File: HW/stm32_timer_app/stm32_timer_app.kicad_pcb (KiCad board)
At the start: 2 copper layers, 121.5 x 72 mm, 30 parts, among them J1 105164-0001, J2 61300411121, J3 PH2-06-UA, Q1 BTA10-600BRG, U1 RT9193-33GB, U2 MOC3041SM, U3 STM32F103C8T6

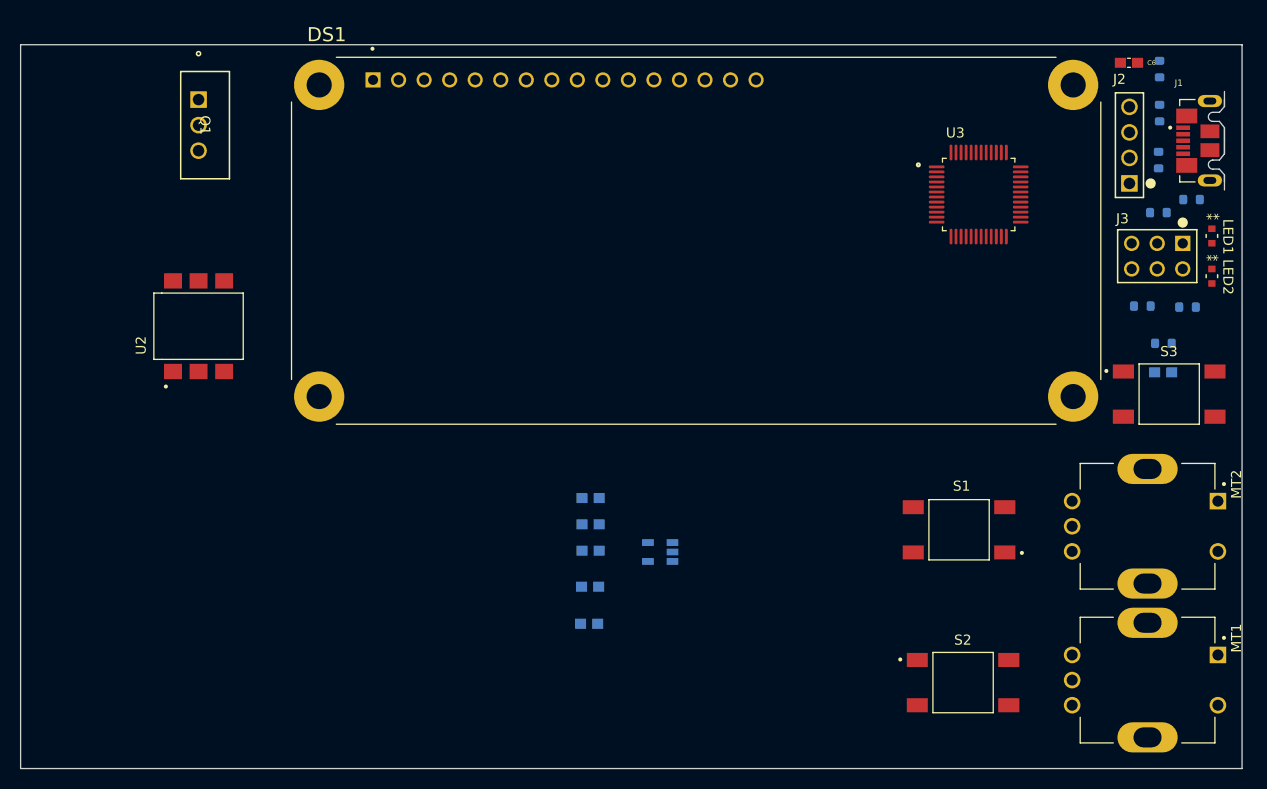
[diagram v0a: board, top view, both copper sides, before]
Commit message: schematic design
schematic design revision 1
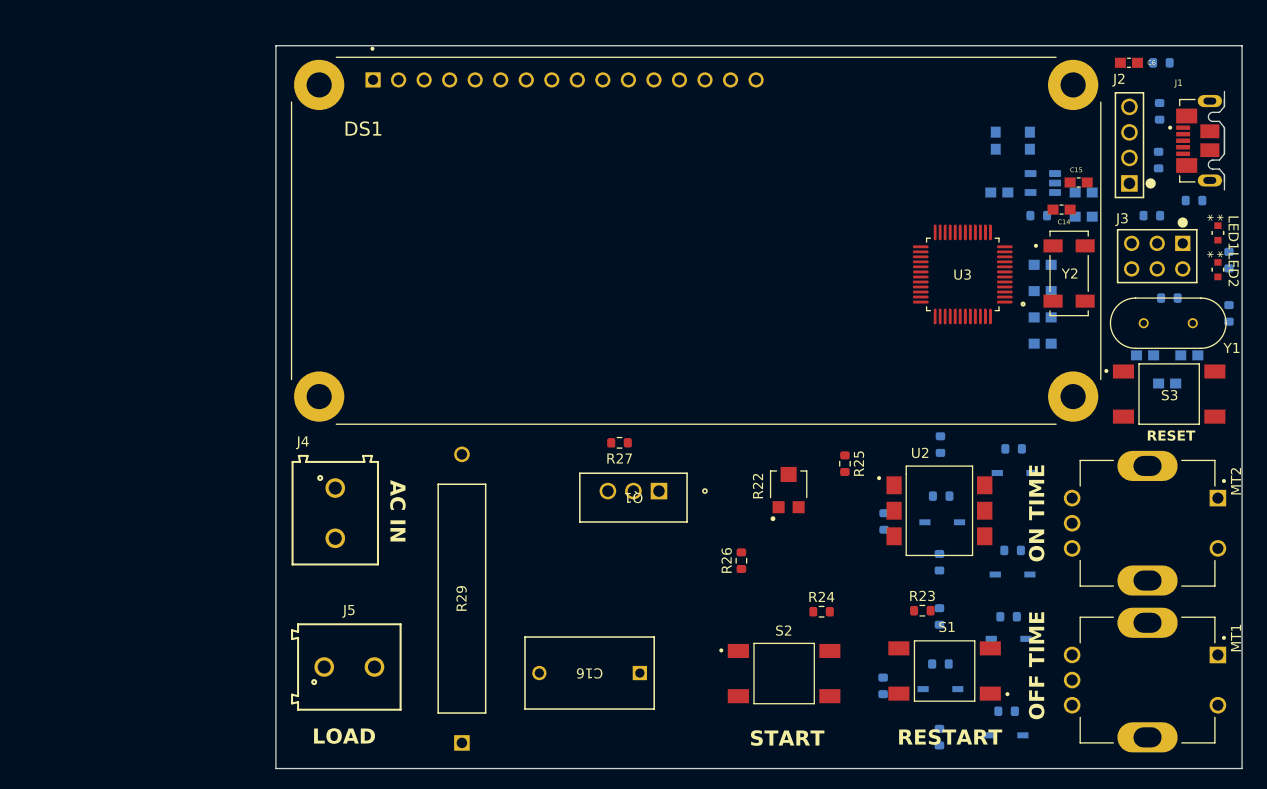
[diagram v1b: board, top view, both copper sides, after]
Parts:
- added C10: 104, LD03ZD475MAB2A:CAPC1608X90, B.Cu at (239.0, 48.1)
- added C11: 104, LD03ZD475MAB2A:CAPC1608X90, B.Cu at (239.0, 50.7)
- added C12: 20p, LD03ZD475MAB2A:CAPC1608X90, B.Cu at (249.2, 51.9)
- added C13: 20p, LD03ZD475MAB2A:CAPC1608X90, B.Cu at (253.6, 51.9)
- added C14: 20p, LD03ZD475MAB2A:CAPC1608X90, F.Cu at (240.8, 37.4)
- added C15: 20p, LD03ZD475MAB2A:CAPC1608X90, F.Cu at (242.6, 34.7)
- added C16: ECW-FD2J273KQ, ECW_FD2J273KQ:CAP_ECWFD_FORMINGQ_12.6LX06.9TX09.9H_PAN, F.Cu at (198.9, 83.5)
- added C8: 104, LD03ZD475MAB2A:CAPC1608X90, B.Cu at (239.0, 42.9)
- added C9: 104, LD03ZD475MAB2A:CAPC1608X90, B.Cu at (239.0, 45.5)
- added CR1: 1N4148W-13-F, 1N4148W_13_F:SOD123_DIO, B.Cu at (235.3, 89.7)
- added CR2: 1N4148W-13-F, 1N4148W_13_F:SOD123_DIO, B.Cu at (235.6, 80.1)
- added CR3: 1N4148W-13-F, 1N4148W_13_F:SOD123_DIO, B.Cu at (228.8, 85.1)
- added CR4: 1N4148W-13-F, 1N4148W_13_F:SOD123_DIO, B.Cu at (236.0, 73.7)
- added CR5: 1N4148W-13-F, 1N4148W_13_F:SOD123_DIO, B.Cu at (236.2, 63.6)
- added CR6: 1N4148W-13-F, 1N4148W_13_F:SOD123_DIO, B.Cu at (229.0, 68.5)
- added J4: 691213710002, 691213710002:691213710002, F.Cu at (168.6, 67.6)
- added J5: 691213710002, 691213710002:691213710002, F.Cu at (170.0, 82.9)
- added R10: 10K, Resistor_SMD:R_0603_1608Metric, B.Cu at (235.4, 87.3)
- added R11: 10K, Resistor_SMD:R_0603_1608Metric, B.Cu at (235.6, 77.9)
- added R12: 10K, Resistor_SMD:R_0603_1608Metric, B.Cu at (228.8, 82.6)
- added R13: 10K, Resistor_SMD:R_0603_1608Metric, B.Cu at (236.1, 61.2)
- added R14: 10K, Resistor_SMD:R_0603_1608Metric, B.Cu at (236.0, 71.3)
- added R15: 10K, Resistor_SMD:R_0603_1608Metric, B.Cu at (228.9, 65.9)
- added R16: 10K, Resistor_SMD:R_0603_1608Metric, B.Cu at (228.7, 89.9)
- added R17: 10K, Resistor_SMD:R_0603_1608Metric, B.Cu at (228.7, 77.9)
- added R18: 10K, Resistor_SMD:R_0603_1608Metric, B.Cu at (223.1, 84.8)
- added R19: 10K, Resistor_SMD:R_0603_1608Metric, B.Cu at (228.7, 72.5)
- added R20: 10K, Resistor_SMD:R_0603_1608Metric, B.Cu at (228.8, 60.8)
- added R21: 10K, Resistor_SMD:R_0603_1608Metric, B.Cu at (223.2, 68.4)
- added R22: TC33X-2-102E, TC33X_2_102E:TRIM_TC33X-2-102E, F.Cu at (213.7, 65.2)
- added R23: 220, Resistor_SMD:R_0603_1608Metric, F.Cu at (227.0, 77.3)
- added R24: 220, Resistor_SMD:R_0603_1608Metric, F.Cu at (217.0, 77.4)
- added R25: 1K, Resistor_SMD:R_0603_1608Metric, F.Cu at (219.3, 62.7)
- added R26: 360, Resistor_SMD:R_0603_1608Metric, F.Cu at (209.0, 72.3)
- added R27: 330, Resistor_SMD:R_0603_1608Metric, F.Cu at (196.9, 60.6)
- added R29: 39, OY390KE:RES_OY_OHM, F.Cu at (181.2, 90.5)
- added R9: 20R, Resistor_SMD:R_0603_1608Metric, B.Cu at (251.6, 46.2)
- added Y1: ABL-8.000MHZ-B2, ABL-8.000MHZ-B2:XTAL_HC49P488W46L1150T500H350, F.Cu at (251.5, 48.7)
- added Y2: ABS25-32.768KHZ-6-4-T, ABS25-32.768KHZ-6-4-T:XTAL_ABS25-32.768KHZ-6-4-T, F.Cu at (241.6, 43.8)
- moved U2 75.9 mm to (228.7, 67.4), turned to 0 degrees
- moved C2 63.7 mm to (243.1, 38.1)
- moved C1 62.8 mm to (243.1, 35.7)
- moved Q1 60.1 mm to (200.8, 65.4), turned to 180 degrees
- moved C4 58.0 mm to (237.7, 30.6), turned to -90 degrees
- moved C5 57.3 mm to (234.3, 30.6), turned to -90 degrees
- moved U1 52.9 mm to (239.0, 34.8)
- moved C3 50.8 mm to (234.7, 35.7), turned to 0 degrees
- moved S2 17.8 mm to (213.2, 83.5)
- moved S1 14.1 mm to (229.2, 83.3)
- moved R6 13.7 mm to (238.6, 38.0)
- moved U3 8.11 mm to (231.0, 43.9), turned to 180 degrees
- moved R4 7.17 mm to (257.5, 47.7), turned to 90 degrees
- moved R8 6.23 mm to (257.5, 42.4), turned to -90 degrees
- moved C7 1.17 mm to (251.3, 54.7)
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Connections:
- C1 pad 2: Net-(U1-EN) -> +5V
- C2 pad 2: Net-(U1-EN) -> +5V
- C4 pad 2: Net-(U1-VOUT) -> PA3
- C5 pad 2: Net-(U1-VOUT) -> PA3
- C6 pad 1: Net-(C6-Pad1) -> PA3
- DS1 pad 1: unconnected-(DS1-VSS-Pad1) -> Net-(DS1-VSS)
- DS1 pad 10: unconnected-(DS1-DB3-Pad10) -> Net-(DS1-DB0)
- DS1 pad 11: unconnected-(DS1-DB4-Pad11) -> PB3
- DS1 pad 12: unconnected-(DS1-DB5-Pad12) -> PB4
- DS1 pad 13: unconnected-(DS1-DB6-Pad13) -> PB5
- DS1 pad 14: unconnected-(DS1-DB7-Pad14) -> PB6
- DS1 pad 15: unconnected-(DS1-VEE-Pad15) -> +5V
- DS1 pad 16: unconnected-(DS1-VEE-Pad16) -> Net-(DS1-DB0)
- DS1 pad 2: unconnected-(DS1-VDD-Pad2) -> +5V
- DS1 pad 3: unconnected-(DS1-VO-Pad3) -> Net-(DS1-VO)
- DS1 pad 4: unconnected-(DS1-RS-Pad4) -> PB1
- DS1 pad 5: unconnected-(DS1-R/~{W}-Pad5) -> Net-(DS1-R/~{W})
- DS1 pad 6: unconnected-(DS1-E-Pad6) -> PB0
- DS1 pad 7: unconnected-(DS1-DB0-Pad7) -> Net-(DS1-DB0)
- DS1 pad 8: unconnected-(DS1-DB1-Pad8) -> Net-(DS1-DB0)
- DS1 pad 9: unconnected-(DS1-DB2-Pad9) -> Net-(DS1-DB0)
- DS1 pad S1: Net-(DS1-SHIELD-PadS1) -> unconnected-(DS1-SHIELD-PadS1)
- DS1 pad S2: Net-(DS1-SHIELD-PadS1) -> unconnected-(DS1-SHIELD-PadS2)
- DS1 pad S3: Net-(DS1-SHIELD-PadS1) -> unconnected-(DS1-SHIELD-PadS3)
- DS1 pad S4: Net-(DS1-SHIELD-PadS1) -> unconnected-(DS1-SHIELD-PadS4)
- J1 pad 5: Net-(J1-Vbus) -> +5V
- J2 pad 1: Net-(C6-Pad1) -> PA3
- J3 pad 5: Net-(J3-Pad5) -> PA3
- J3 pad 6: Net-(J3-Pad5) -> PA3
- LED1 pad 2: Net-(LED1-Pad2) -> PA3
- LED2 pad 2: Net-(LED1-Pad2) -> PA3
- MT1 pad 1: unconnected-(MT1-Pad1) -> Net-(MT1-Pad1)
- MT1 pad 2: unconnected-(MT1-Pad2) -> Net-(CR1-Pad2)
- MT1 pad A: unconnected-(MT1-PadA) -> Net-(CR2-Pad2)
- MT1 pad B: unconnected-(MT1-PadB) -> Net-(CR3-Pad2)
- MT1 pad COM: unconnected-(MT1-PadCOM) -> Net-(MT1-Pad1)
- MT1 pad S1: Net-(MT1-SHIELD-PadS1) -> Net-(MT1-Pad1)
- MT1 pad S2: Net-(MT1-SHIELD-PadS1) -> Net-(MT1-Pad1)
- MT2 pad 1: unconnected-(MT2-Pad1) -> Net-(MT2-Pad1)
- MT2 pad 2: unconnected-(MT2-Pad2) -> Net-(CR4-Pad2)
- MT2 pad A: unconnected-(MT2-PadA) -> Net-(CR5-Pad2)
- MT2 pad B: unconnected-(MT2-PadB) -> Net-(CR6-Pad2)
- MT2 pad COM: unconnected-(MT2-PadCOM) -> Net-(MT2-Pad1)
- MT2 pad S1: Net-(MT2-SHIELD-PadS1) -> Net-(MT2-Pad1)
- MT2 pad S2: Net-(MT2-SHIELD-PadS1) -> Net-(MT2-Pad1)
- Q1 pad 1: unconnected-(Q1-A1-Pad1) -> Net-(Q1-A1)
- Q1 pad 2: unconnected-(Q1-A2-Pad2) -> Net-(Q1-A2)
- Q1 pad 3: unconnected-(Q1-G-Pad3) -> Net-(Q1-G)
- R3 pad 1: Net-(R3-Pad1) -> +5V
- R4 pad 2: Net-(R4-Pad2) -> PA3
- S1 pad 3: Net-(S1-Pad3) -> PA3
- S1 pad 4: Net-(S1-Pad3) -> PA3
- S2 pad 3: Net-(S2-Pad3) -> PA3
- S2 pad 4: Net-(S2-Pad3) -> PA3
- U1 pad 1: Net-(U1-EN) -> +5V
- U1 pad 3: Net-(U1-EN) -> +5V
- U1 pad 5: Net-(U1-VOUT) -> PA3
- U2 pad 1: unconnected-(U2-Pad1) -> Net-(R25-Pad2)
- U2 pad 2: unconnected-(U2-Pad2) -> Net-(U2-Pad2)
- U2 pad 4: unconnected-(U2-Pad4) -> Net-(Q1-G)
- U2 pad 6: unconnected-(U2-Pad6) -> Net-(R26-Pad1)
- U3 pad 10: unconnected-(U3-PA0_WKUP-Pad10) -> PA0
- U3 pad 11: unconnected-(U3-PA1-Pad11) -> PA1
- U3 pad 12: unconnected-(U3-PA2-Pad12) -> PA2
- U3 pad 13: unconnected-(U3-PA3-Pad13) -> PA3
- U3 pad 14: unconnected-(U3-PA4-Pad14) -> PA3
- U3 pad 15: unconnected-(U3-PA5-Pad15) -> PA5
- U3 pad 16: unconnected-(U3-PA6-Pad16) -> PA6
- U3 pad 17: unconnected-(U3-PA7-Pad17) -> PA7
- U3 pad 18: unconnected-(U3-PB0-Pad18) -> PB0
- U3 pad 19: unconnected-(U3-PB1-Pad19) -> PB1
- U3 pad 24: Net-(U3-VDD-Pad24) -> PA3
- U3 pad 3: unconnected-(U3-PC14-OSC32_IN-Pad3) -> PC14
- U3 pad 36: unconnected-(U3-VDD-Pad36) -> PA3
- U3 pad 39: unconnected-(U3-PB3-Pad39) -> PB3
- U3 pad 4: unconnected-(U3-PC15-OSC32_OUT-Pad4) -> PC15
- U3 pad 40: unconnected-(U3-PB4-Pad40) -> PB4
- U3 pad 41: unconnected-(U3-PB5-Pad41) -> PB5
- U3 pad 42: unconnected-(U3-PB6-Pad42) -> PB6
- U3 pad 43: unconnected-(U3-PB7-Pad43) -> PB7
- U3 pad 48: unconnected-(U3-VDD-Pad48) -> PA3
- U3 pad 5: unconnected-(U3-PD0_OSC_IN-Pad5) -> OSCIN
- U3 pad 6: unconnected-(U3-PD1_OSC_OUT-Pad6) -> OSCOUT
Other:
- board size 121.5 x 72 mm -> 96.1 x 71.9 mm
- board text added: "AC IN"
- board text added: "LOAD"
- board text added: "OFF TIME"
- board text added: "ON TIME"
- board text added: "RESET"
- board text added: "RESTART"
- board text added: "START"
